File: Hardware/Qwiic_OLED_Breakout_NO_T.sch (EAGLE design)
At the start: 26 parts

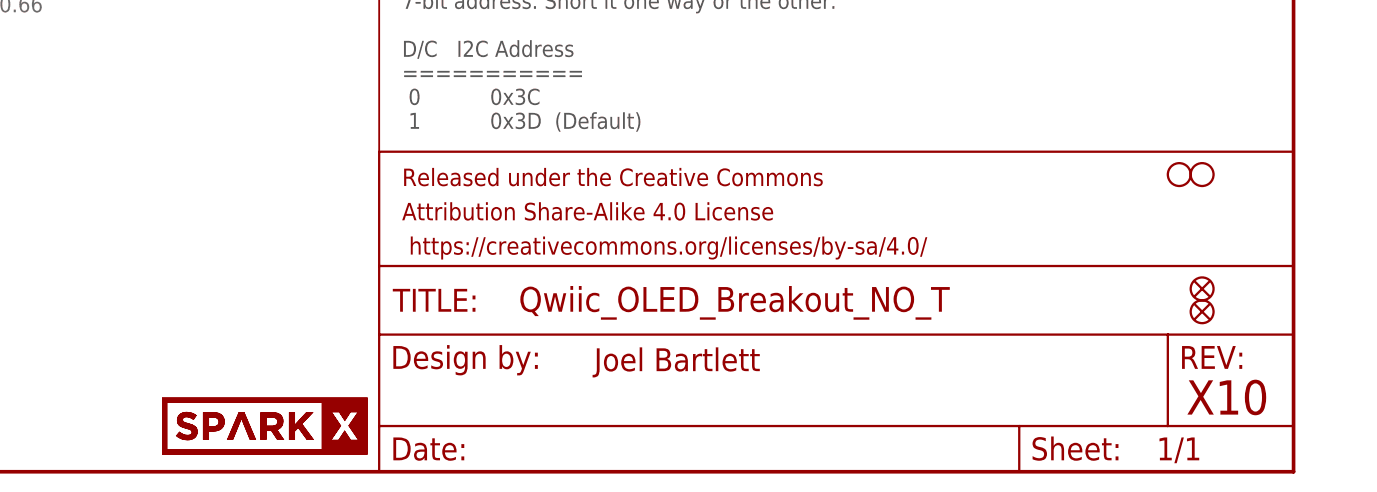
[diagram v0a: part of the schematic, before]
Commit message: Adding Gerbers
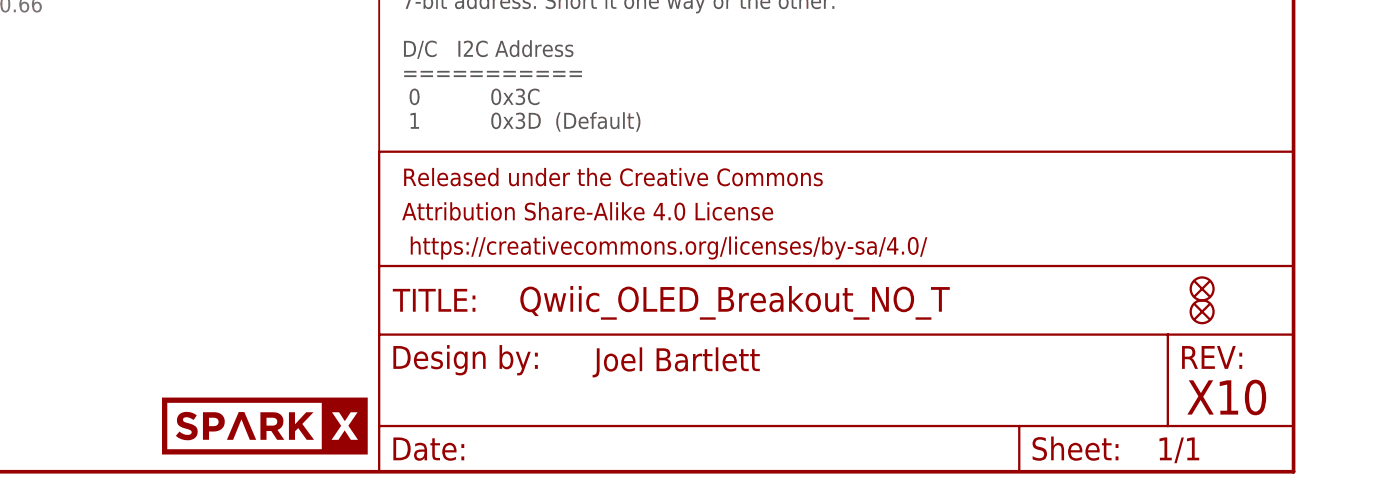
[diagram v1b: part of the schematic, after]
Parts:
- removed H1, H2: STAND-OFF, SparkFun-Hardware:STAND-OFF
- removed U$1: SPARKX-LOGO4, SparkX:SPARKX-LOGO4
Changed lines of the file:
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@@
 <part name="SUPPLY7" library="SparkFun-Aesthetics" deviceset="VDD" device=""/>
 <part name="GND13" library="SparkFun-Aesthetics" deviceset="GND" device=""/>
-<part name="U$1" library="SparkX" deviceset="SPARKX-LOGO" device="4" value="SPARKX-LOGO4"/>
 <part name="R3" library="SparkFun-Passives" deviceset="RESISTOR" device="0603-RES" value="10k"/>
 <part name="SUPPLY8" library="SparkFun-Aesthetics" deviceset="VDD" device=""/>
@@
 <part name="R14" library="SparkFun-Resistors" deviceset="4.7KOHM" device="-0603-1/10W-1%" value="4.7k"/>
 <part name="JP2" library="SparkFun-Jumpers" deviceset="JUMPER-SMT_3_2-NC_PASTE" device="_SILK" value=""/>
-<part name="H1" library="SparkFun-Hardware" deviceset="STAND-OFF" device=""/>
-<part name="H2" library="SparkFun-Hardware" deviceset="STAND-OFF" device=""/>
 <part name="SUPPLY2" library="SparkFun-Aesthetics" deviceset="VDD" device=""/>
 <part name="JP3" library="SparkFun-Jumpers" deviceset="JUMPER-SMT_2_NO" device="_SILK" value=""/>
@@
 <instance part="SUPPLY7" gate="VDD" x="25.4" y="93.98"/>
 <instance part="GND13" gate="1" x="25.4" y="78.74"/>
-<instance part="U$1" gate="G$1" x="134.62" y="5.08"/>
 <instance part="R3" gate="G$1" x="157.48" y="88.9" rot="MR90"/>
 <instance part="SUPPLY8" gate="VDD" x="157.48" y="96.52" rot="MR0"/>
@@
 <instance part="R14" gate="G$1" x="68.58" y="147.32" rot="R90"/>
 <instance part="JP2" gate="G$1" x="60.96" y="157.48" rot="R270"/>
-<instance part="H1" gate="G$1" x="236.22" y="33.02"/>
-<instance part="H2" gate="G$1" x="238.76" y="33.02"/>
 <instance part="SUPPLY2" gate="VDD" x="60.96" y="165.1"/>
 <instance part="JP3" gate="G$1" x="157.48" y="71.12" rot="R90"/>
